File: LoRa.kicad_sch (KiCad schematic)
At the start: 1 part, among them IC1 114993390

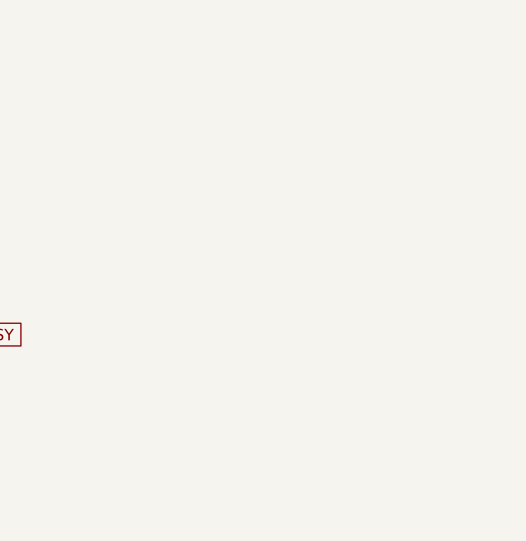
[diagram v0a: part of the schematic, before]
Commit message: Finished preliminary project schematics and architecture
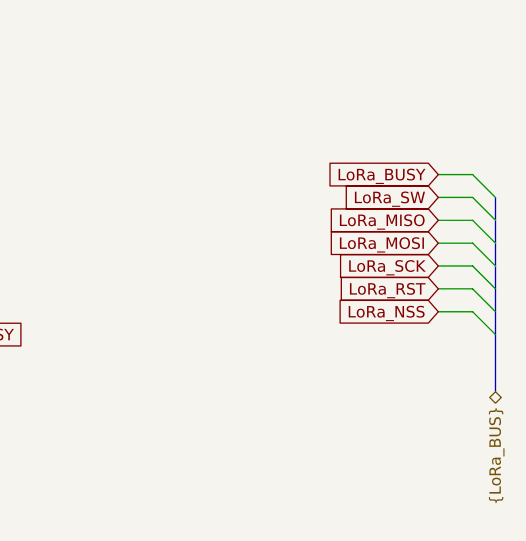
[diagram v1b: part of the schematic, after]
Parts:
- IC1: footprint Project_Components:114993390 -> 00_lora:wio-sx1262
